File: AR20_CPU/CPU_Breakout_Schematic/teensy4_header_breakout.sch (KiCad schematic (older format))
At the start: 19 parts, among them J1 Conn_01x05, J2 Conn_01x14, J3 Micro_SD_Card, J4 Conn_01x14, SW1 SW_SPST, U2 MCP2551-I-SN

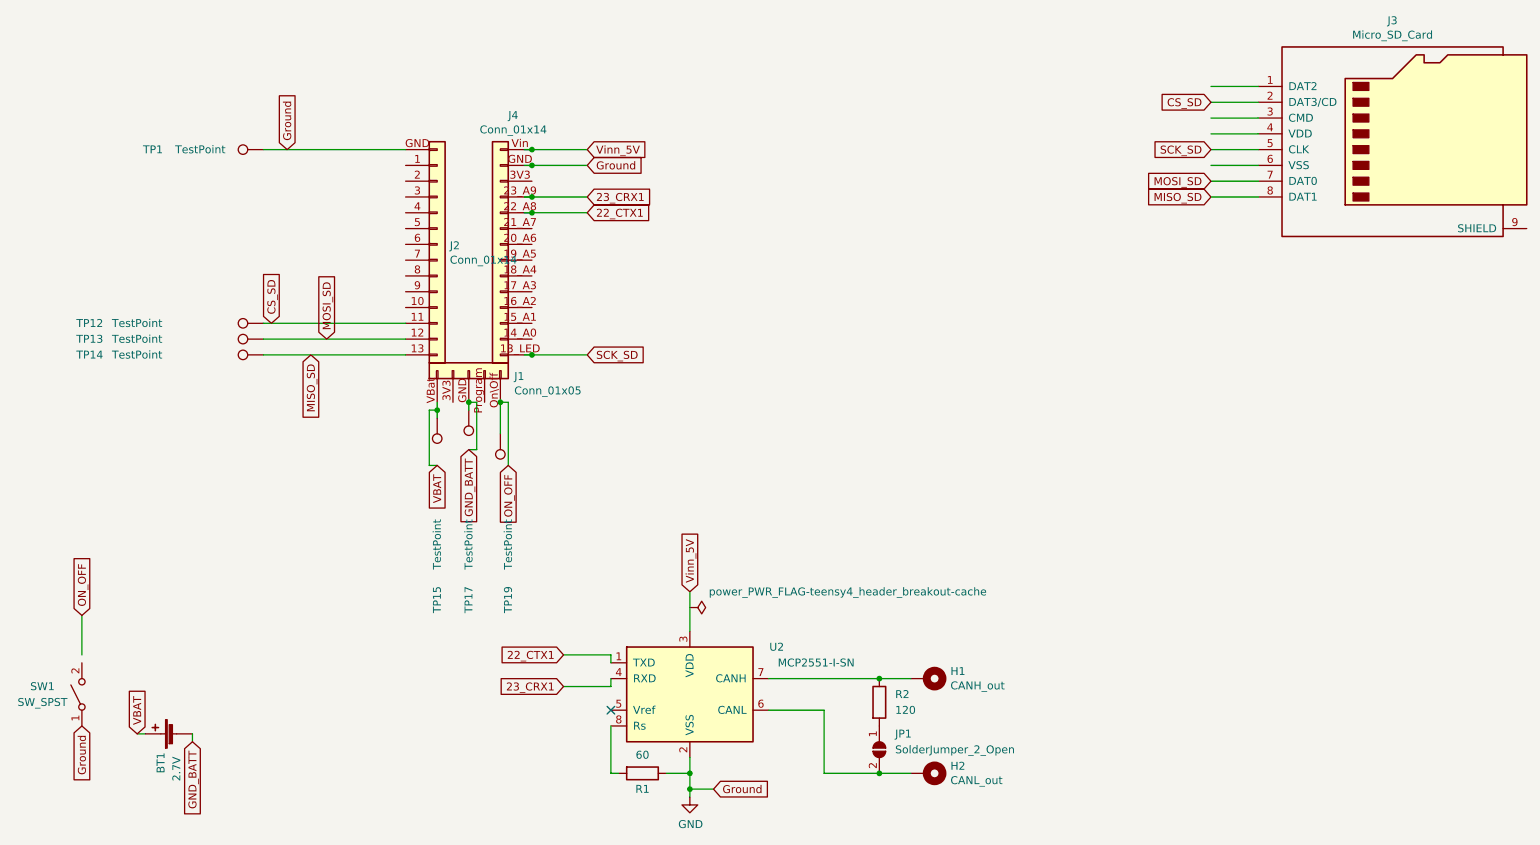
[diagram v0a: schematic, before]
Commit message: Edited test points
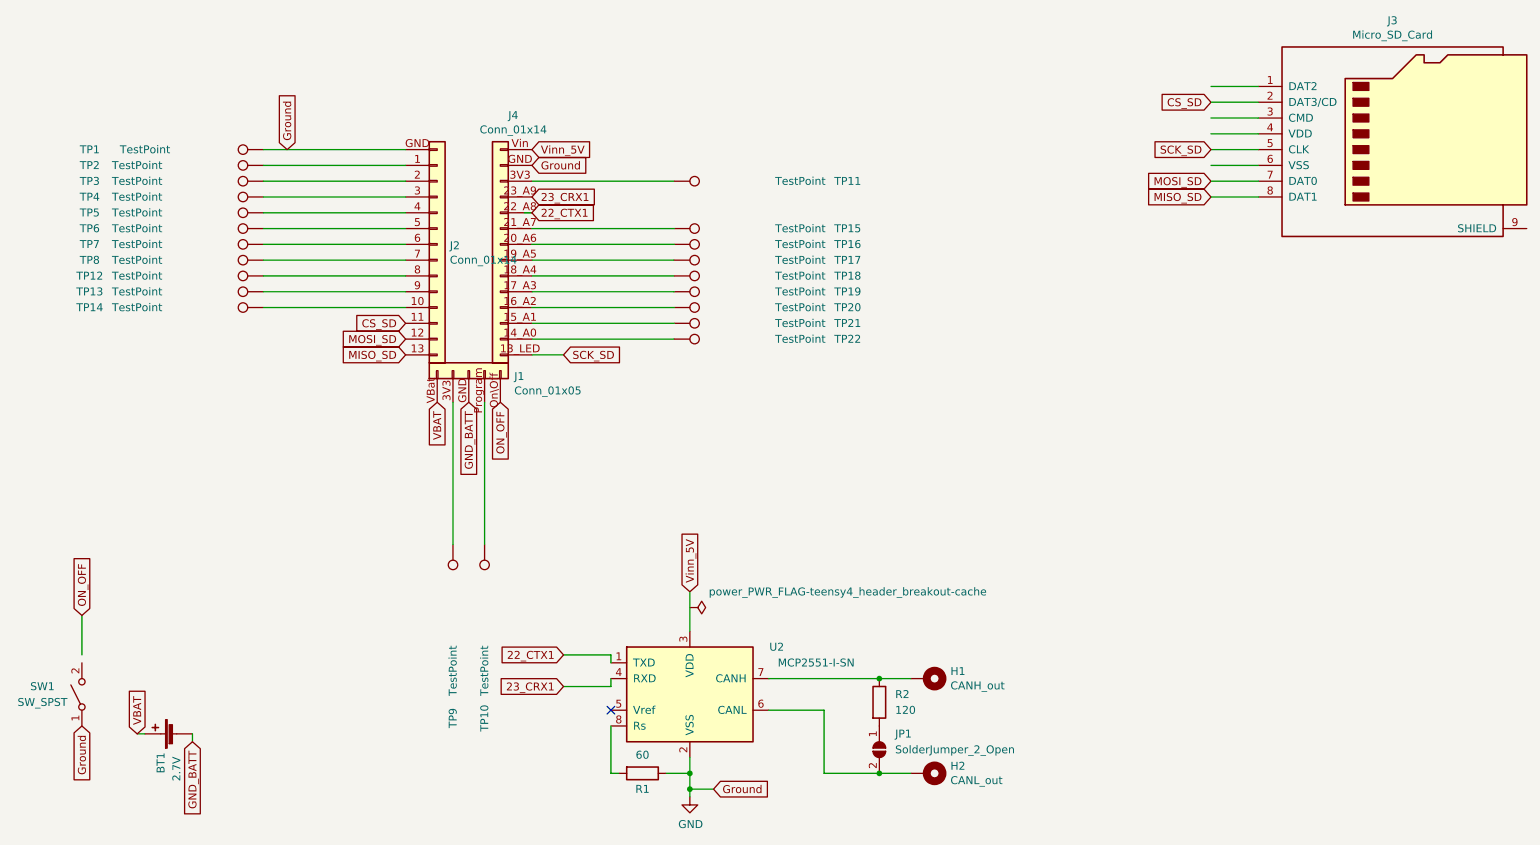
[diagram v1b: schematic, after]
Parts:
- added TP10, TP11, TP16, TP18, TP2, TP20, TP21, TP22, TP3, TP4, TP5, TP6, TP7, TP8, TP9: TestPoint, TestPoint:TestPoint_THTPad_D1.0mm_Drill0.5mm, symbol Connector:TestPoint
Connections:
- wire segments 55 -> 53
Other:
- moved on the sheet: TP12, TP13, TP14
